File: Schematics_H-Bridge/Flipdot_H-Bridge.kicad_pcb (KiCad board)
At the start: 2 copper layers, 100 x 100 mm, 76 parts, among them J1 Barrel_Jack, P1 CONN_02X13, P2 CONN_02X08, P3 CONN_02X08, P4 CONN_02X03, SW1 SW_Push, U1 74HC595, U10 L293D, U11 L293D, U12 L293D, U13 74HC595, U14 L293D, U15 L293D, U16 L293D, U17 L293D, U18 L293D, U19 L293D, U2 74HC595, U20 ESP8266_D1_Mini, U21 L293D, U22 L293D, U23 L293D, U24 L293D, U25 L293D, U26 L293D, U27 L7805, U28 ATMEGA328P-PU, U3 L293D, U4 L293D, U5 L293D, U6 L293D, U7 74HC595, U8 74HC595, U9 L293D, Y1 Crystal

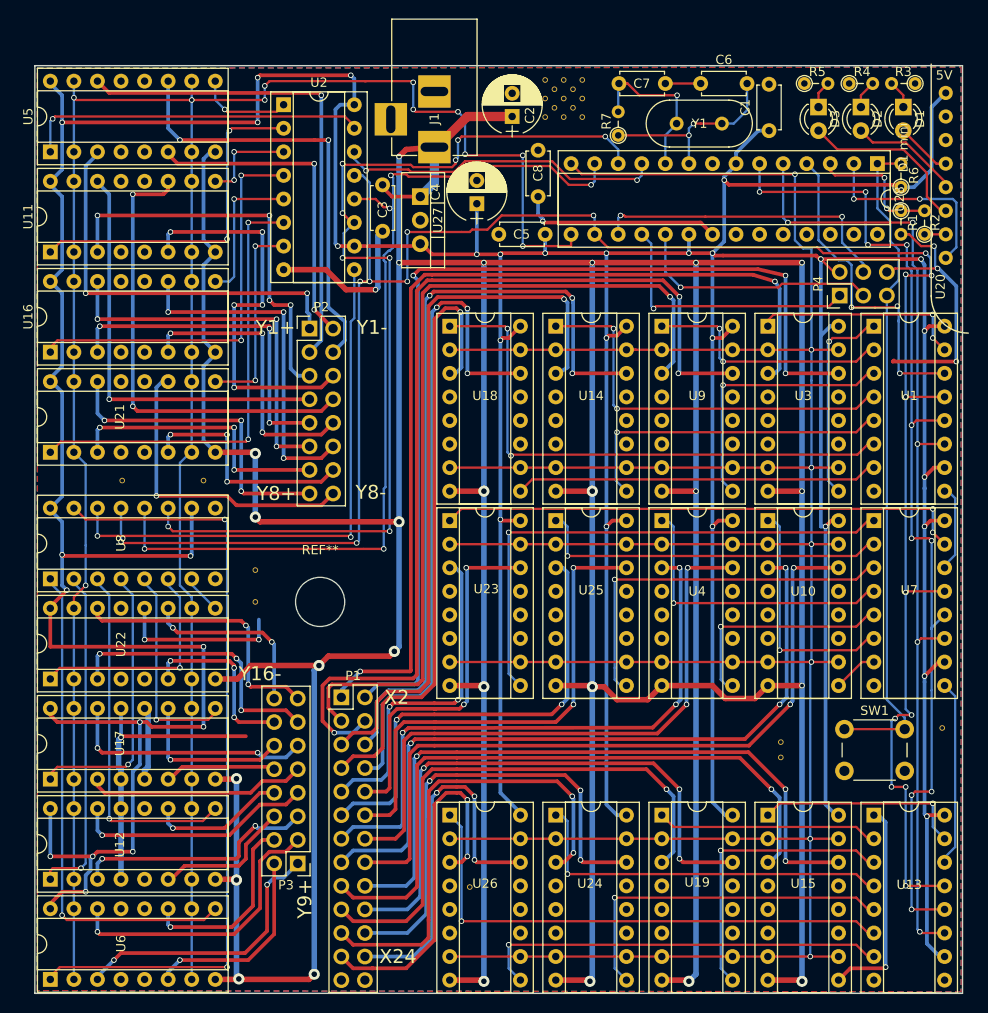
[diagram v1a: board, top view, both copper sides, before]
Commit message: PCB v1.1, minor fixes in connector and silkscreen layout
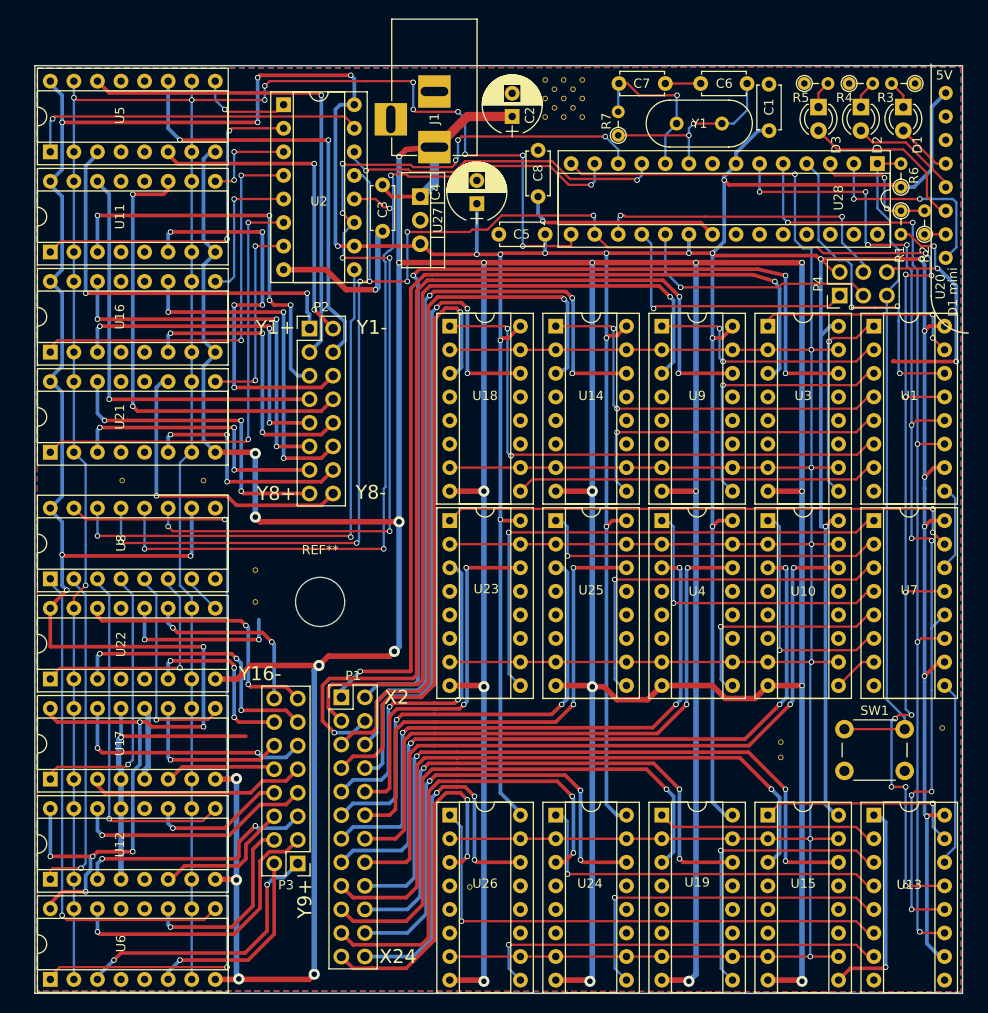
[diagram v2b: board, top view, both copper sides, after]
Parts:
- P1: footprint Pin_Headers:Pin_Header_Straight_2x13_Pitch2.54mm -> Pin_Headers:Pin_Header_Straight_2x12_Pitch2.54mm

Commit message: removed old ESP code
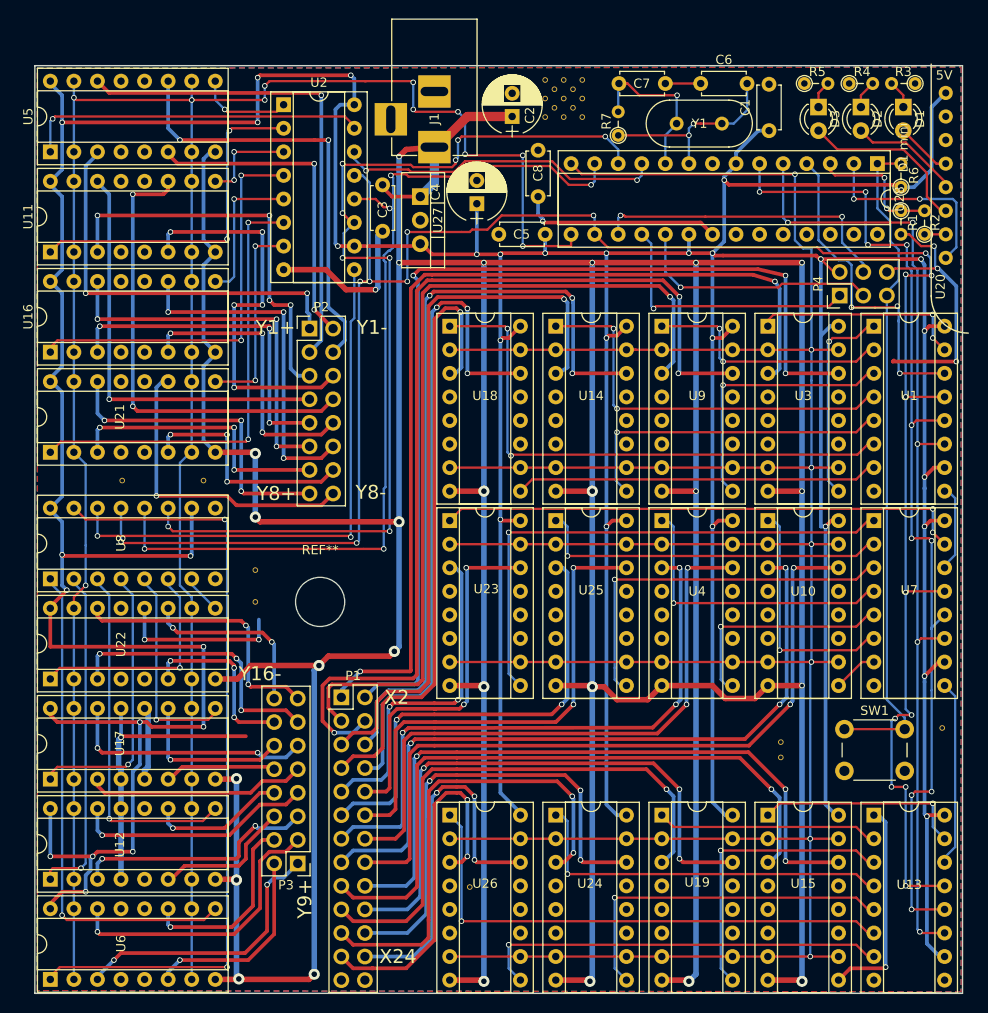
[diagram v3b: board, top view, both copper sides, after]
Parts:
- P1: footprint Pin_Headers:Pin_Header_Straight_2x12_Pitch2.54mm -> Pin_Headers:Pin_Header_Straight_2x13_Pitch2.54mm
